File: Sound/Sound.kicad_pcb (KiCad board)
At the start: 4 copper layers, 133.6 x 74.7 mm, 31 parts, among them J1 2x19 2.54mm Right-angled Head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, U1 74HCT74, U2 74HCT02, U3 74HCT138, U4 74HCT138, U5 LM386, U6 LM386, U7 LM386

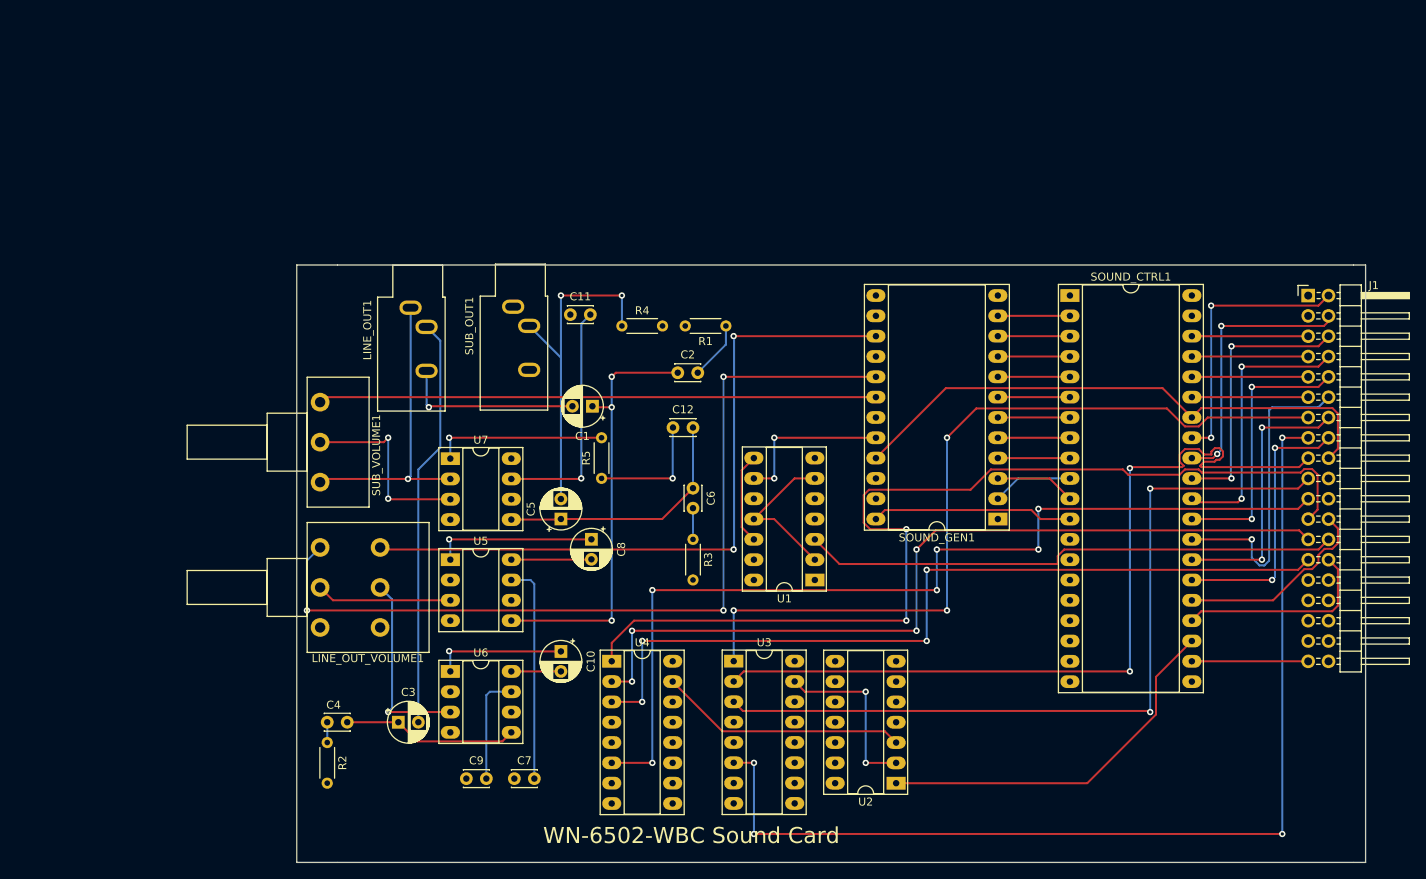
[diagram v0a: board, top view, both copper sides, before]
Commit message: Updated worksheet...
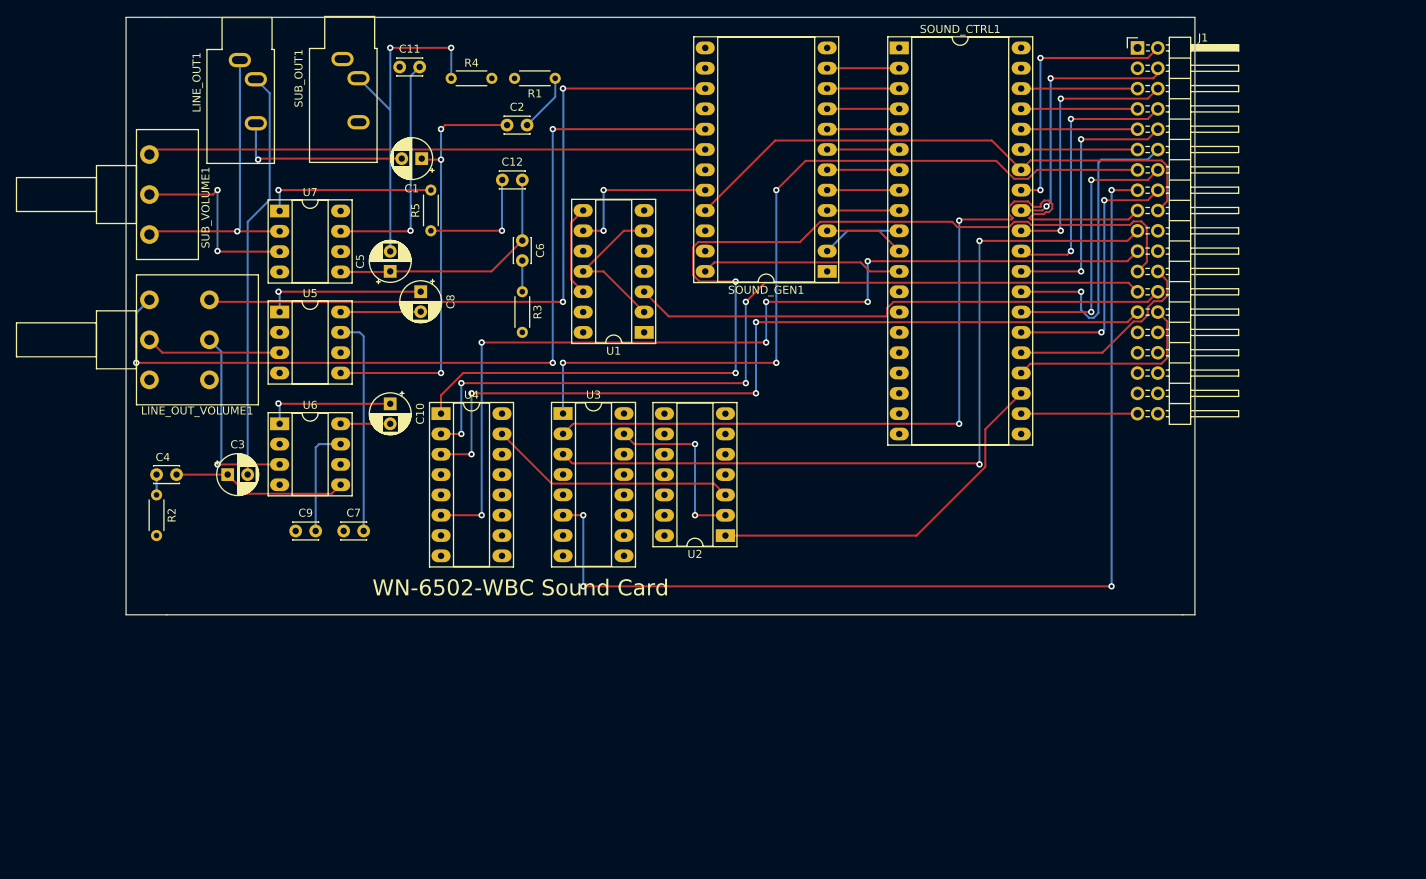
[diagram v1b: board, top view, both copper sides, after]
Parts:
- moved R5 37.6 mm to (67.6, 46.5)
- moved C1 37.6 mm to (66.4, 37.5)
- moved C11 37.6 mm to (63.7, 26.0)
- moved C12 37.6 mm to (76.5, 40.2)
- moved C2 37.6 mm to (77.1, 33.3)
- moved C3 37.6 mm to (42.2, 77.0)
- moved C4 37.6 mm to (35.8, 77.0)
- moved C6 37.6 mm to (79.0, 47.7)
- moved C8 37.6 mm to (66.3, 54.1)
- moved LINE_OUT1 37.6 mm to (43.7, 25.2)
- moved R1 37.6 mm to (83.1, 27.5)
- moved R3 37.6 mm to (79.0, 54.1)
- moved R4 37.6 mm to (70.1, 27.5)
- moved SOUND_CTRL1 37.6 mm to (126.1, 23.7)
- moved SOUND_GEN1 37.6 mm to (117.1, 51.6)
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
